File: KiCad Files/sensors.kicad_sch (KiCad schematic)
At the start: 0 parts

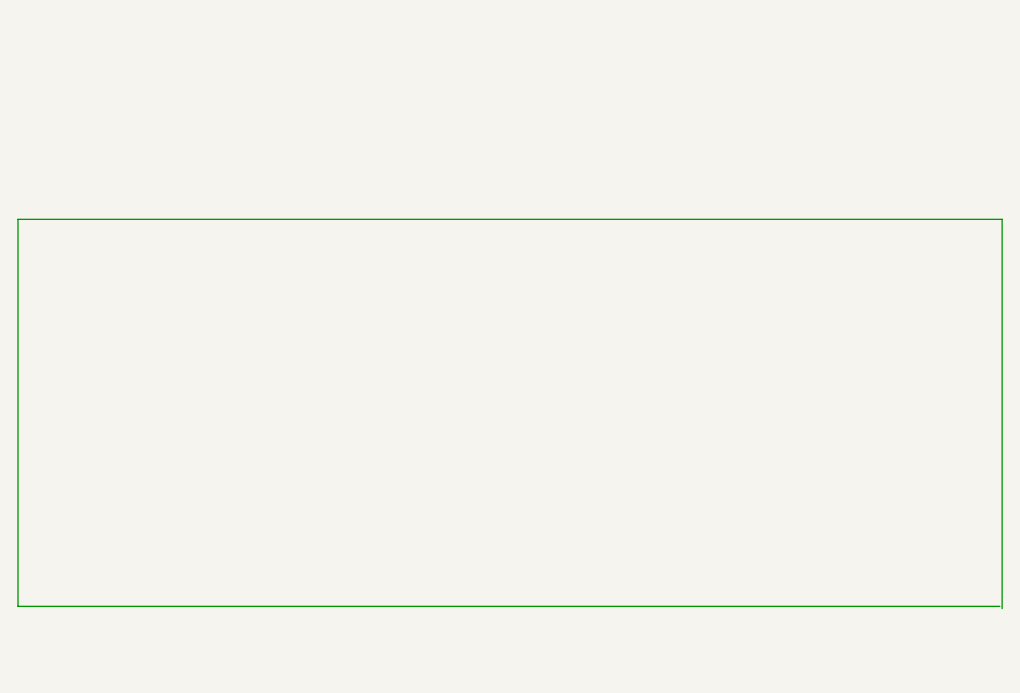
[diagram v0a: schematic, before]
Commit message: hall1
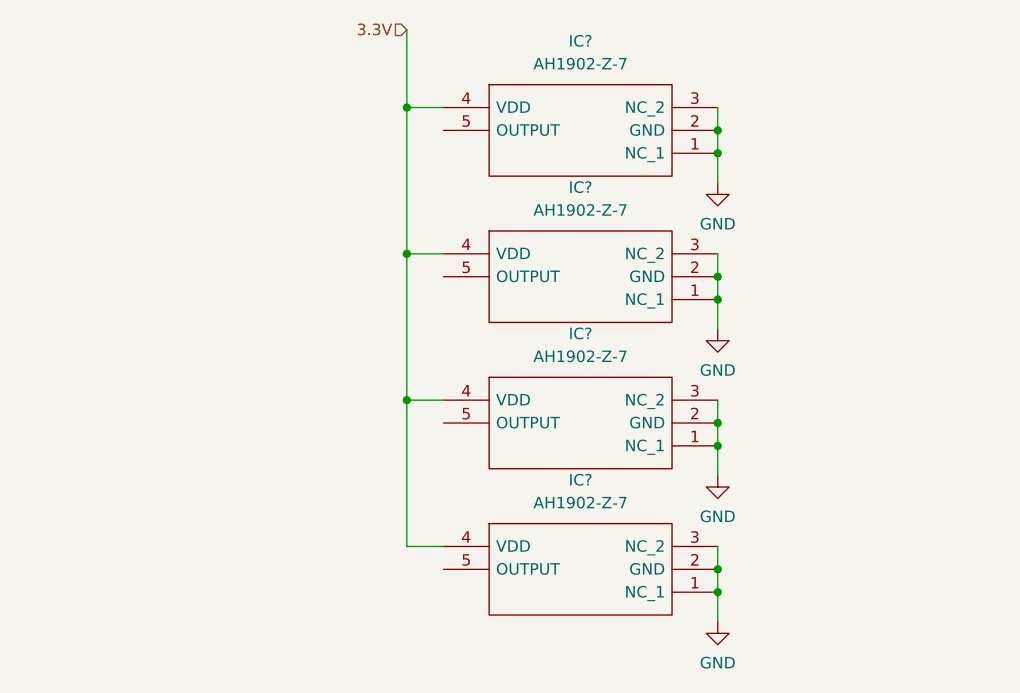
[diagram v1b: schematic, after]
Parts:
- added IC? (x4): AH1902-Z-7, AH1902Z7, symbol AH1902-Z-7:AH1902-Z-7
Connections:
- new net 3.3V: IC?.4 (VDD), IC?.4 (VDD), IC?.4 (VDD), IC?.4 (VDD)
- new net GND: IC?.1 (NC_1), IC?.1 (NC_1), IC?.1 (NC_1), IC?.1 (NC_1), IC?.2 (GND), IC?.2 (GND), IC?.2 (GND), IC?.2 (GND), IC?.3 (NC_2), IC?.3 (NC_2), IC?.3 (NC_2), IC?.3 (NC_2)
